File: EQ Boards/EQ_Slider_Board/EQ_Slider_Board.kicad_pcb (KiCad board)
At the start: 2 copper layers, 111.8 x 63.5 mm, 26 parts

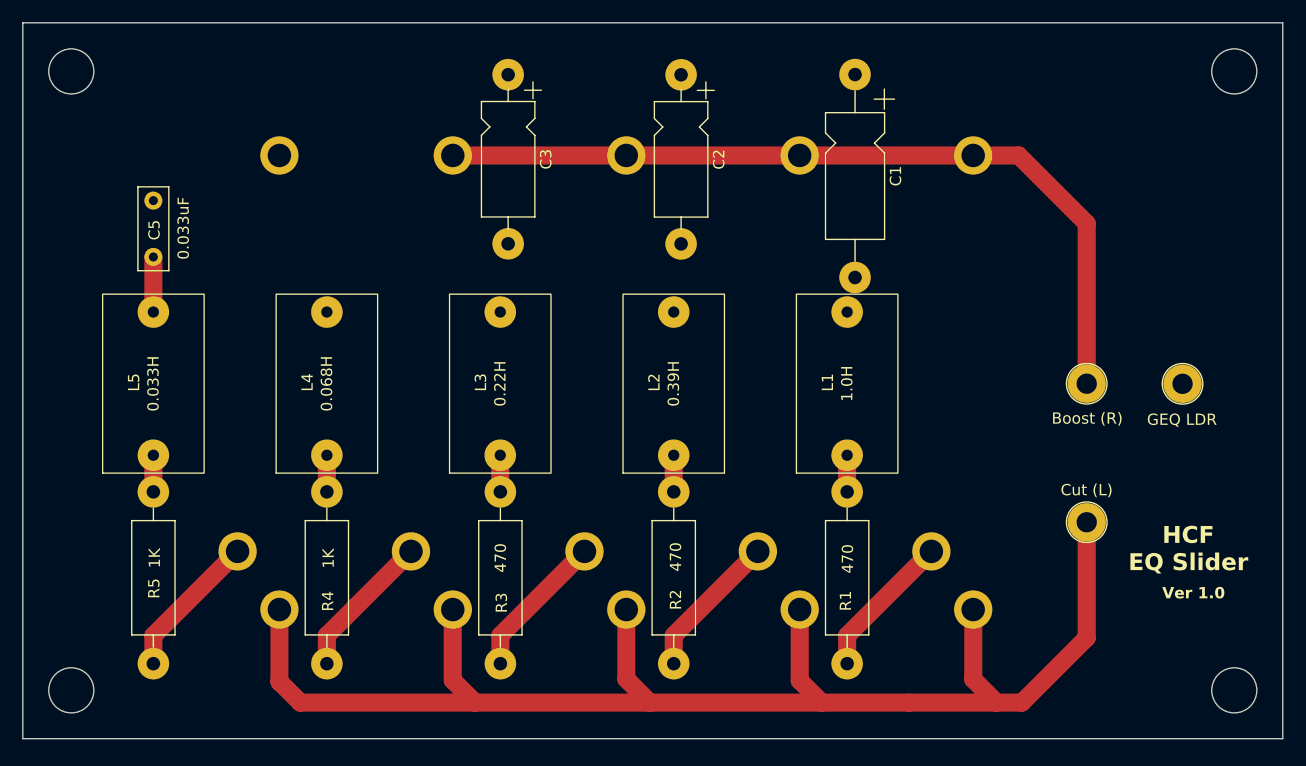
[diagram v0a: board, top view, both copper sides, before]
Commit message: Finished EQ Slider V1 Board
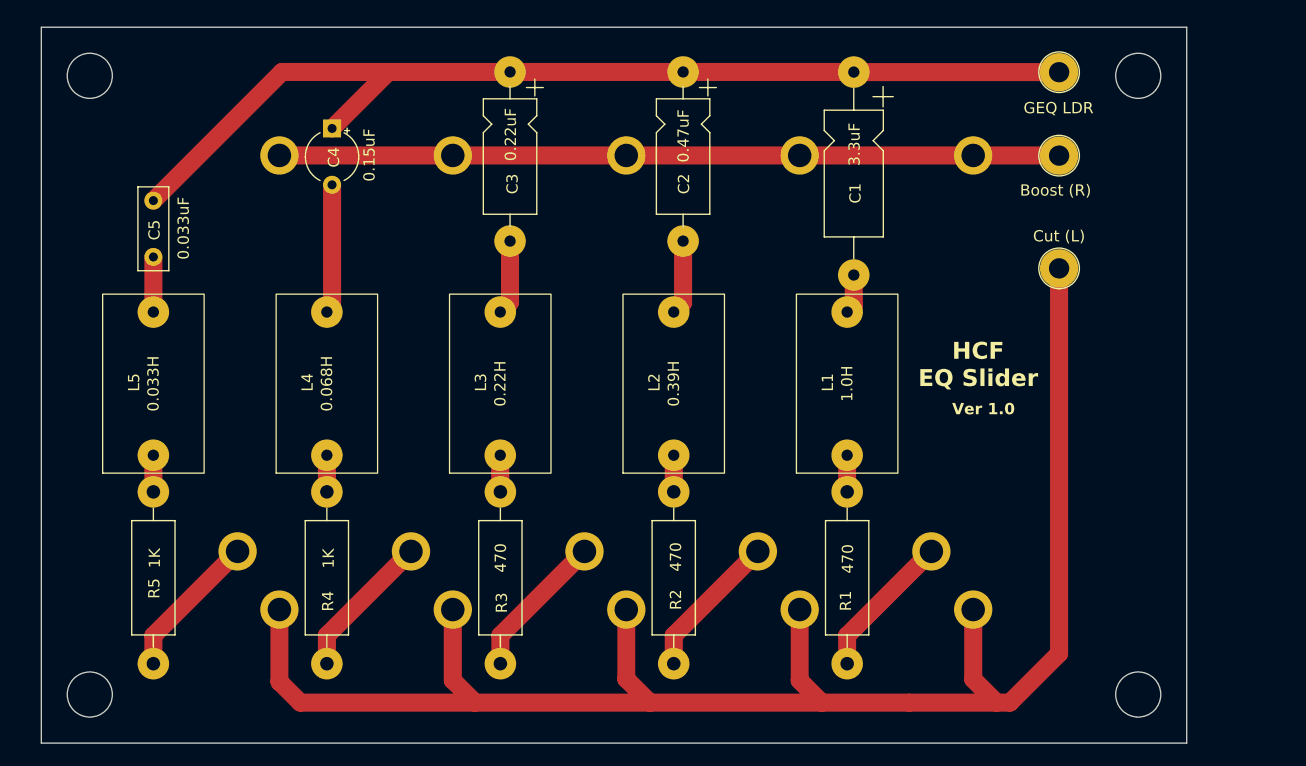
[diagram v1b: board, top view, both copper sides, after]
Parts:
- added C4: 0.15uF, Capacitor_THT:CP_Radial_Tantal_D4.5mm_P5.00mm, F.Cu at (131.3, 75.8)
- moved TP3 29.7 mm to (195.8, 70.8)
- moved TP1 22.7 mm to (195.8, 88.2)
- moved TP2 20.4 mm to (195.8, 78.2)
- moved REF** 8.53 mm to (202.8, 71.2)
- moved REF** 8.53 mm to (202.8, 126.0)
- moved REF** 1.69 mm to (109.8, 71.2)
- moved REF** 1.68 mm to (109.8, 126.0)
- moved C2 0.31 mm to (162.4, 70.8)
- moved C3 0.29 mm to (147.1, 70.8)
- moved C1 0.25 mm to (177.6, 70.8)
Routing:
- net Net-(C1-Pad1): track 0.00 -> 92.2 mm
- net Net-(RV1-Pad3): track 127.8 -> 148.7 mm
- net Net-(C4-Pad2): track 0.00 -> 11.5 mm
- net Net-(C3-Pad2): track 0.00 -> 6.65 mm
- net Net-(C2-Pad2): track 0.00 -> 6.64 mm
- net Net-(RV1-Pad1): track 72.9 -> 69.2 mm
- net Net-(C1-Pad2): track 0.00 -> 3.53 mm
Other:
- board size 111.8 x 63.5 mm -> 101.6 x 63.5 mm
